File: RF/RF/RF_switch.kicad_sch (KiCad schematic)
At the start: 6 parts, among them IC401 PE4250MLI-Z

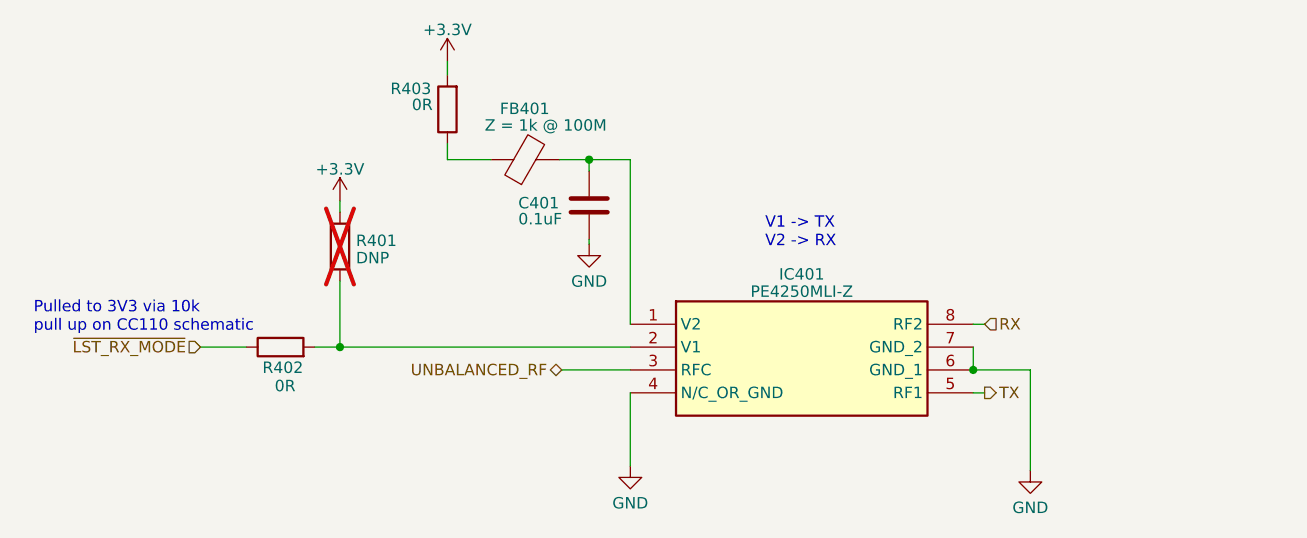
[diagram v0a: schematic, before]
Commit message: RF: Push for schematic capture review version 1.0
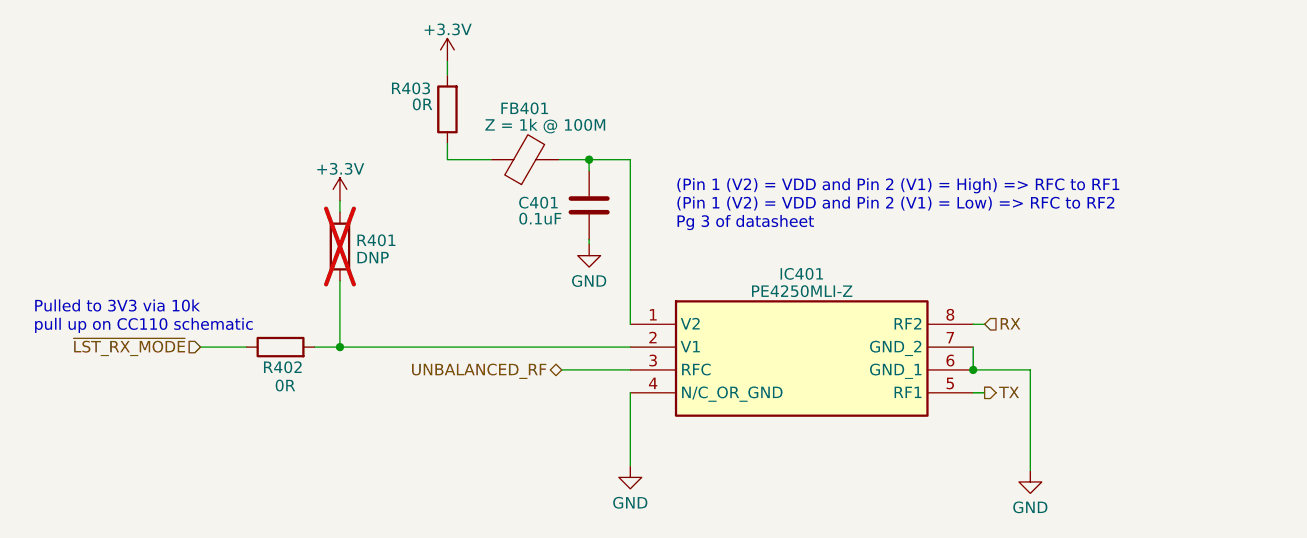
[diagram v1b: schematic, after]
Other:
- note added: "(Pin 1 (V2) = VDD and Pin 2 (V1) = High) => RFC to RF1 (Pin 1 (V2) = VDD and Pin 2 (V1) = Low) => RFC to RF2 Pg 3 of datasheet"
- note removed: "V1 -> TX V2 -> RX"
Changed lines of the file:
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@@
     (effects (font (size 1.27 1.27)) (justify left bottom))
   )
-  (text "V1 -> TX\nV2 -> RX" (at 148.336 69.596 0)
+  (text "(Pin 1 (V2) = VDD and Pin 2 (V1) = High) => RFC to RF1\n(Pin 1 (V2) = VDD and Pin 2 (V1) = Low) => RFC to RF2\nPg 3 of datasheet"
+    (at 138.43 67.564 0)
     (effects (font (size 1.27 1.27)) (justify left bottom))
   )
